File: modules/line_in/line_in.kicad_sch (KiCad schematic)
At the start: 24 parts, among them J2 Outputs, U1 LM358, U2 LM358, U3 LM358

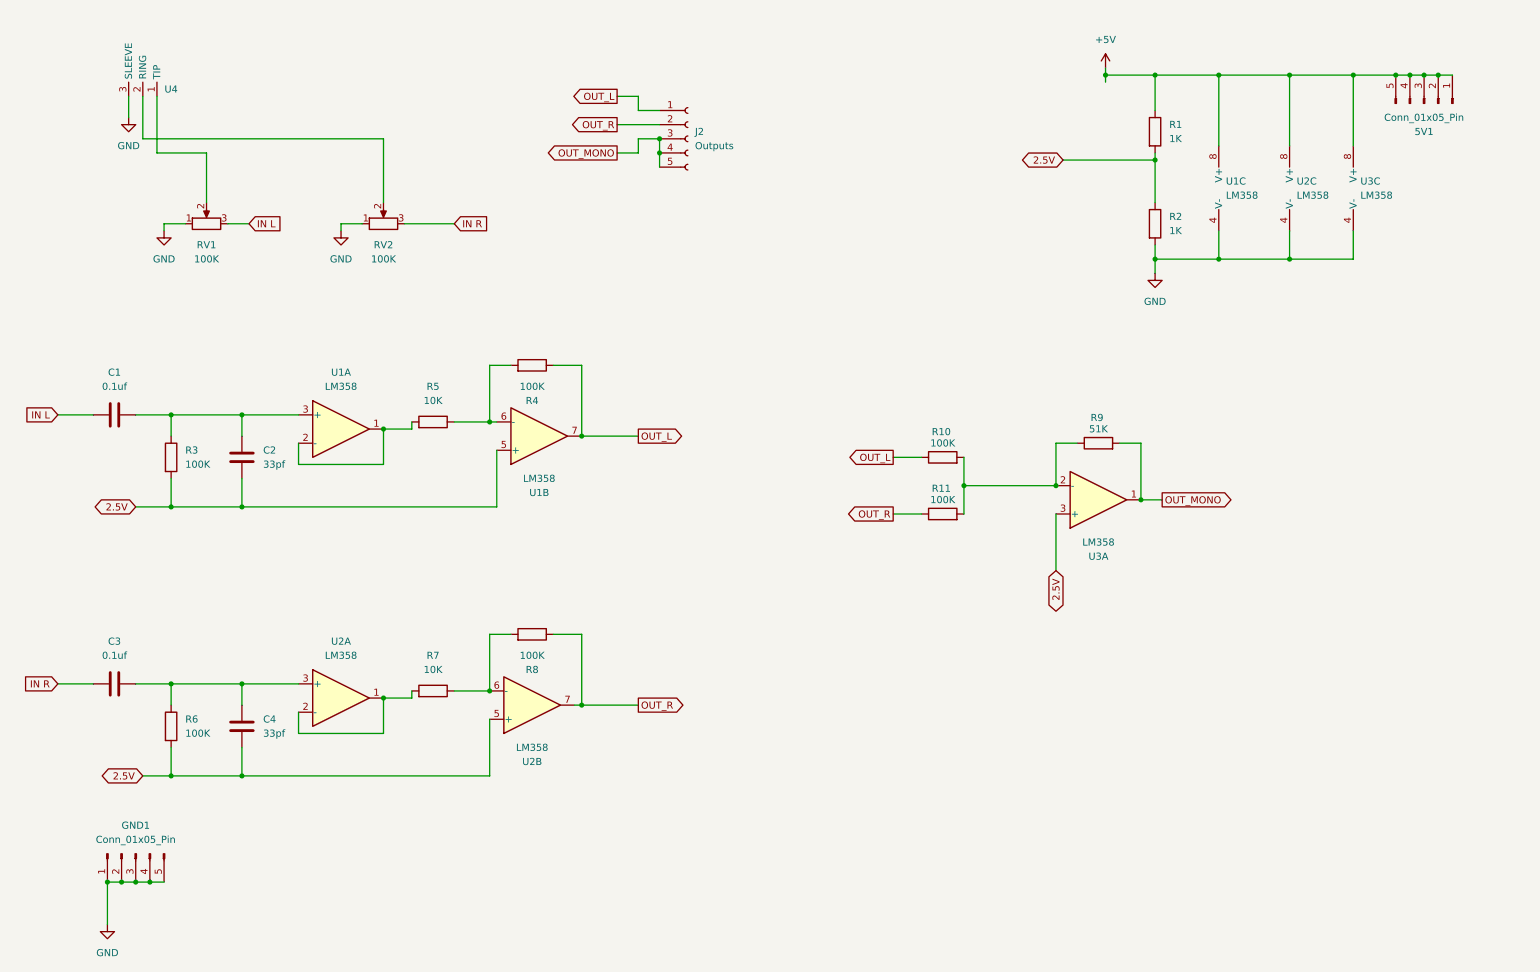
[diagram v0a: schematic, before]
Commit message: Start working on the new version of line_in
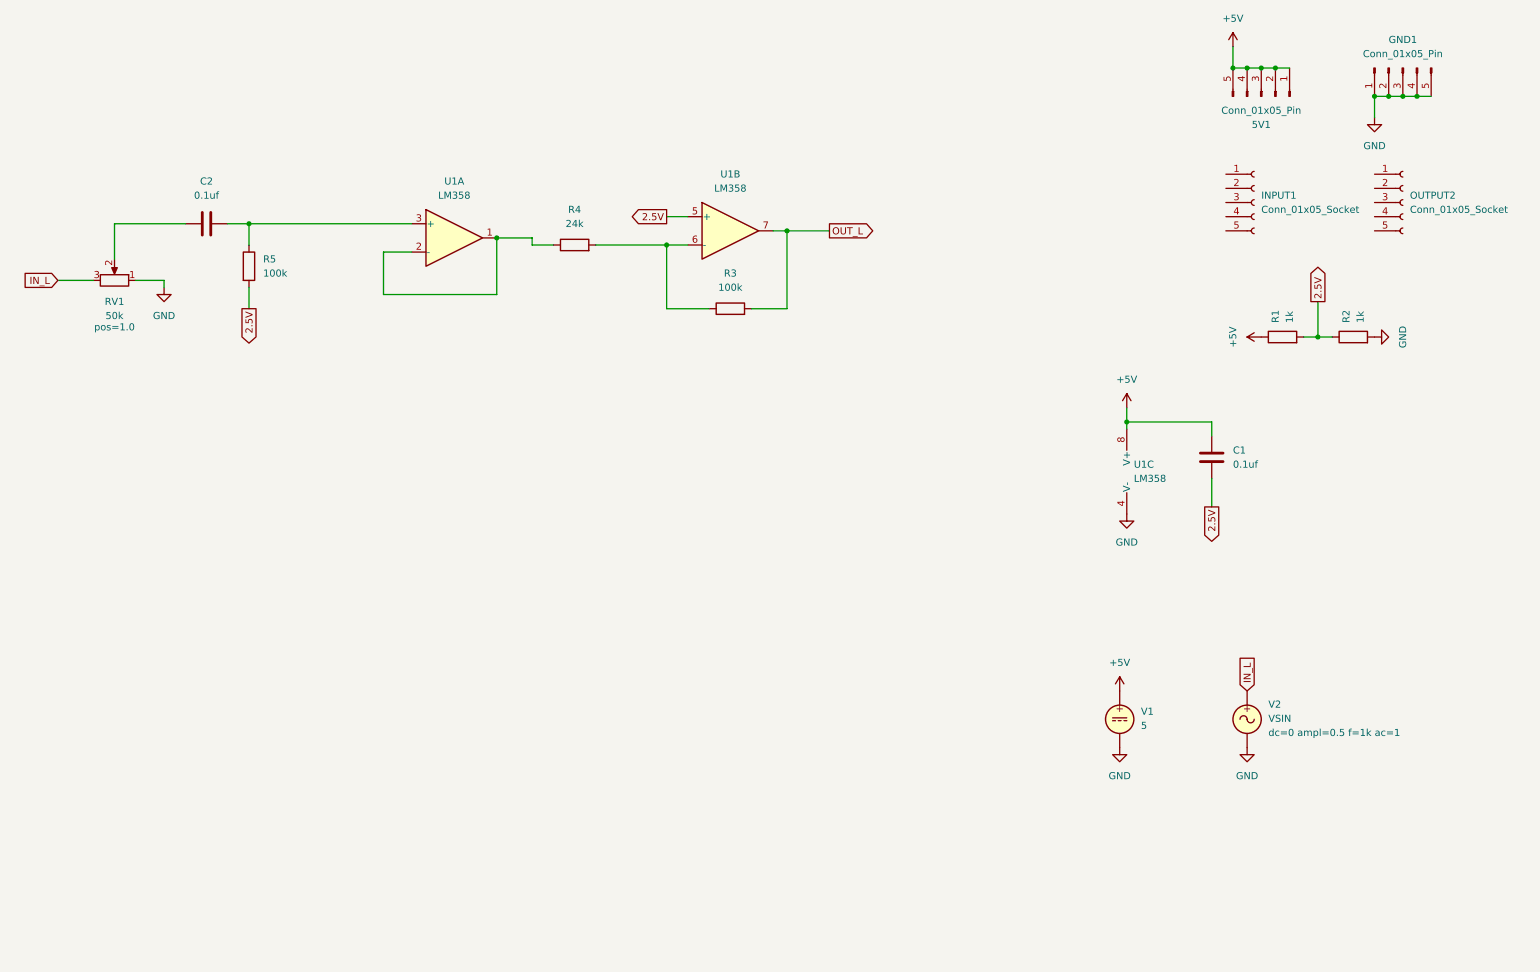
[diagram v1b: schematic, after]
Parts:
- removed C3: 0.1uf, Capacitor_SMD:C_0402_1005Metric, symbol Device:C
- removed C4: 33pf, Capacitor_SMD:C_0402_1005Metric, symbol Device:C
- removed J2: Outputs, Connector_PinSocket_2.54mm:PinSocket_1x05_P2.54mm_Vertical, symbol Connector:Conn_01x05_Socket
- removed R10, R11, R6, R8: 100K, Resistor_SMD:R_0402_1005Metric, symbol Device:R
- removed R7: 10K, Resistor_SMD:R_0402_1005Metric, symbol Device:R
- removed R9: 51K, Resistor_SMD:R_0402_1005Metric, symbol Device:R
- removed RV2: 100K, Potentiometer_THT:Potentiometer_Alpha_RD901F-40-00D_Single_Vertical, symbol Device:R_Potentiometer
- removed U2, U3: LM358, Package_SO:SOIC-8-1EP_3.9x4.9mm_P1.27mm_EP2.29x3mm, symbol Amplifier_Operational:LM358
- removed U4: ~, Footprints:Audio_Socket_TRS_3.5mm, symbol Symbols:Audio_Jack_TRS_3.5mm
- added INPUT1, OUTPUT2: Conn_01x05_Socket, Connector_PinSocket_2.54mm:PinSocket_1x05_P2.54mm_Vertical, symbol Connector:Conn_01x05_Socket
- added V1: 5, symbol Simulation_SPICE:VDC
- added V2: VSIN, symbol Simulation_SPICE:VSIN
- C1: footprint Capacitor_SMD:C_0402_1005Metric -> (none)
- C2: value 33pf -> 0.1uf; footprint Capacitor_SMD:C_0402_1005Metric -> (none)
- R1, R2: value 1K -> 1k; footprint Resistor_SMD:R_0402_1005Metric -> (none)
- R3: value 100K -> 100k; footprint Resistor_SMD:R_0402_1005Metric -> (none)
- R4: value 100K -> 24k; footprint Resistor_SMD:R_0402_1005Metric -> (none)
- R5: value 10K -> 100k; footprint Resistor_SMD:R_0402_1005Metric -> (none)
- RV1: value 100K -> 50k; footprint Potentiometer_THT:Potentiometer_Alpha_RD901F-40-00D_Single_Vertical -> (none)
- U1: footprint Package_SO:SOIC-8-1EP_3.9x4.9mm_P1.27mm_EP2.29x3mm -> (none)
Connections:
- net +5V: now also C1.1, V1.1
- net 2.5V: now also C1.2, R5.2; no longer C2.2, R3.2
- net GND: now also V1.2, V2.2
- net OUT_L: now also R3.2; no longer R4.1
- net at R4.2, U1.6 (-): now also R3.1; no longer R5.1
- net at U1.1, U1.2 (-): now also R4.1; no longer R5.2
- net at RV1.2: now also C2.1
- net IN L renamed IN_L
- net IN_L: now also V2.1; no longer C1.2
- new net: C2.2, R5.1, U1.3 (+)
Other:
- moved on the sheet: 5V1, GND1
